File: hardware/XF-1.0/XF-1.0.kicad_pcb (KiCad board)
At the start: 2 copper layers, 121.3 x 99.7 mm, 16 parts

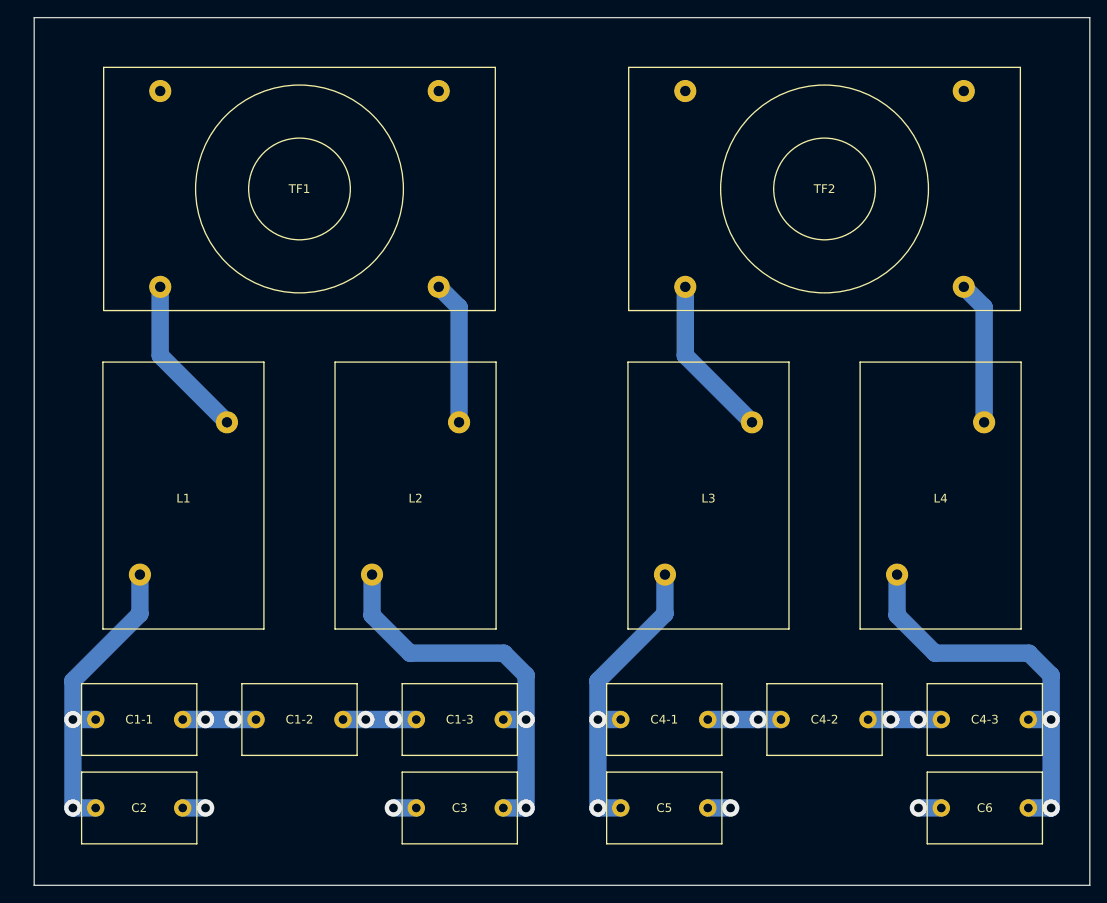
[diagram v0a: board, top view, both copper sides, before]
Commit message: modified:   Ferrite Transformer Calculation.xlsx 	modified:   README.md 	deleted:    hardware/XF-1.0/XF-1.0-backups/XF-1.0-2025-07-15_095716.zip 	new file:   hardware/XF-1.0/XF-1.0-backups/XF-1.0-2025-07-15_145509.zip 	new file:   hardware/XF-1.0/XF-1.0-backups/XF-1.0-2025-07-15_150114.zip 	new file:   hardware/XF-1.0/XF-1.0-backups/XF-1.0-2025-07-15_150614.zip 	new file:   hardware/XF-1.0/XF-1.0-backups/XF-1.0-2025-07-15_151503.zip 	new file:   hardware/XF-1.0/XF-1.0-backups/XF-1.0-2025-07-15_152320.zip 	new file:   hardware/XF-1.0/XF-1.0-backups/XF-1.0-2025-07-15_154638.zip 	modified:   hardware/XF-1.0/XF-1.0.kicad_pcb 	modified:   hardware/XF-1.0/XF-1.0.kicad_prl 	modified:   hardware/XF-1.0/XF-1.0.kicad_pro 	modified:   hardware/XF-1.0/XF-1.0.kicad_sch 	modified:   hardware/XF-1.0/_autosave-XF-1.0.kicad_sch 	modified:   hardware/XF-1.0/fp-info-cache
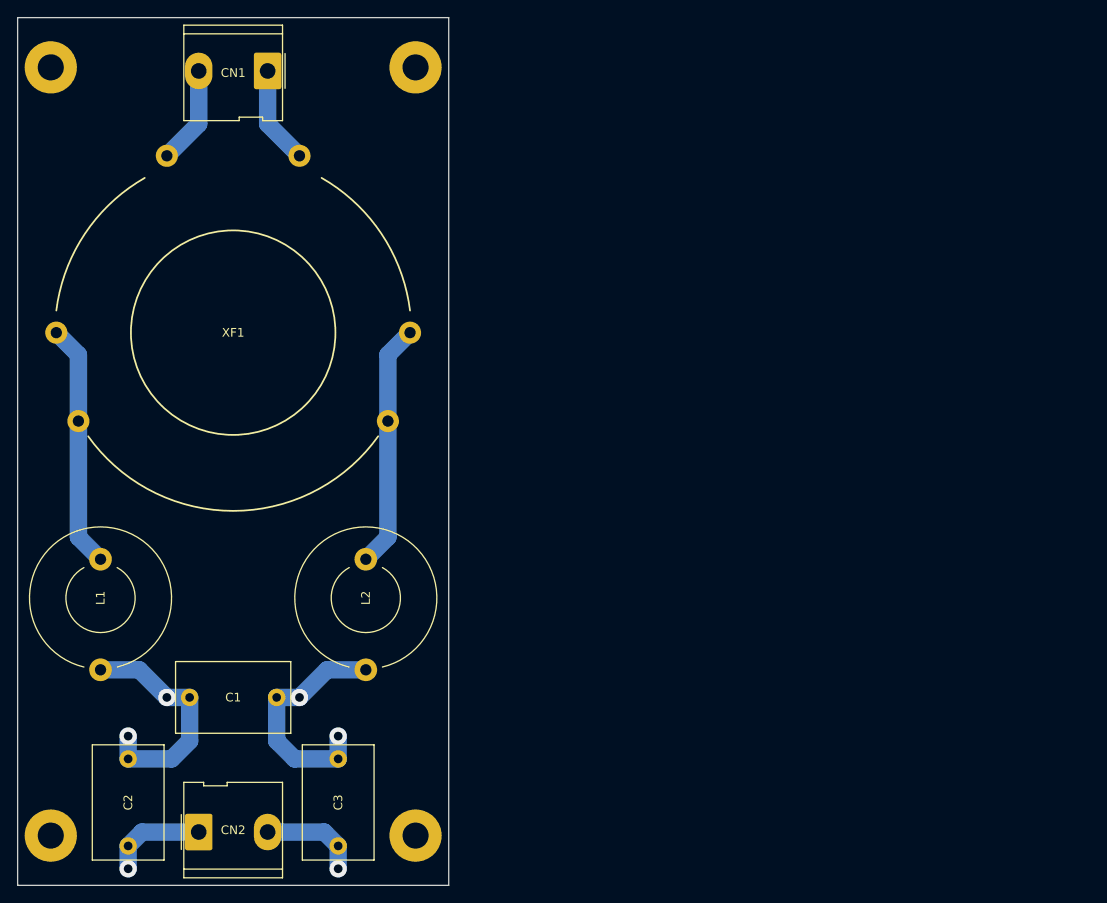
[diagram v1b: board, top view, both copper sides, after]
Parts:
- removed C1-1, C1-2, C1-3, C4-1, C4-2, C4-3: 1nF, Capacitor_THT:C_Rect_L13.0mm_W8.0mm_P10.00mm_FKS3_FKP3_MKS4
- removed C5, C6: 4.7nF, Capacitor_THT:C_Rect_L13.0mm_W8.0mm_P10.00mm_FKS3_FKP3_MKS4
- removed L3, L4: ~, Transformer_THT:Inductor-EE25
- removed TF1, TF2: ~, Transformer_THT:EE35-1P-1S-Vertical-2143
- added C1: 2.7nF, Capacitor_THT:C_Rect_L13.0mm_W8.0mm_P10.00mm_FKS3_FKP3_MKS4, F.Cu at (43.3, 124.5)
- added CN1: Conn_01x02, Connector_Molex:Molex_KK-396_5273-03A_1x03_P3.96mm_Vertical_2, F.Cu at (52.2, 52.5)
- added CN2: Conn_01x02, Connector_Molex:Molex_KK-396_5273-03A_1x03_P3.96mm_Vertical_2, F.Cu at (44.3, 139.9)
- added H1: ~, MountingHole:MountingHole_3mm_Pad, F.Cu at (27.3, 52.1)
- added H2: ~, MountingHole:MountingHole_3mm_Pad, F.Cu at (69.2, 52.1)
- added H3: ~, MountingHole:MountingHole_3mm_Pad, F.Cu at (27.3, 140.3)
- added H4: ~, MountingHole:MountingHole_3mm_Pad, F.Cu at (69.2, 140.3)
- added XF1: ~, Transformer_THT:Transformer_Toroid_Horizontal_OD40_ID23_H15, F.Cu at (48.3, 82.5)
- L1, L2: value ~ -> 29µH; footprint Transformer_THT:Inductor-EE25 -> Inductor_THT:L_Radial_Multilayer_D8.0mm_P12.70mm
- moved C3 19.8 mm to (60.3, 131.5), turned to -90 degrees
- moved L1 14.9 mm to (33.0, 113.0), turned to -90 degrees
- moved L2 12.8 mm to (63.5, 113.0), turned to -90 degrees
- moved C2 6.76 mm to (36.2, 131.5), turned to -90 degrees
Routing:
- net Net-(C4-3-Pad2): track 45.7 -> 0.00 mm, vias 2 -> 0
- net Net-(C4-1-Pad1): track 35.2 -> 0.00 mm, vias 2 -> 0
- net Net-(L3-Pad1): track 18.7 -> 0.00 mm
- net Net-(C1-Pad2): track 45.7 -> 27.1 mm
- net Net-(L4-Pad1): track 16.5 -> 0.00 mm
- net Net-(L2-Pad1): track 16.5 -> 28.1 mm
- net Net-(CN1-Pin_1): track 0.00 -> 11.3 mm
- net Net-(CN1-Pin_2): track 0.00 -> 11.3 mm
- net Net-(L1-Pad1): track 18.7 -> 28.1 mm
- net Net-(CN2-Pin_2): track 2.62 -> 11.4 mm
- net Net-(CN2-Pin_1): track 2.62 -> 11.4 mm
- net Net-(C4-2-Pad2): track 8.42 -> 0.00 mm, vias 2 -> 0
- net Net-(C1-2-Pad2): track 8.41 -> 0.00 mm, vias 2 -> 0
- net Net-(C1-1-Pad2): track 8.41 -> 0.00 mm, vias 2 -> 0
- net Net-(C4-1-Pad2): track 8.41 -> 0.00 mm, vias 2 -> 0
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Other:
- board size 121.3 x 99.7 mm -> 49.5 x 99.7 mm

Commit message: modified:   Ferrite Transformer Calculation.xlsx 	modified:   README.md 	deleted:    hardware/CTL-1.0/CTL-1.0-backups/CTL-1.0-2025-05-28_203223.zip 	new file:   hardware/CTL-1.0/CTL-1.0-backups/CTL-1.0-2025-07-16_143147.zip 	deleted:    hardware/PS-2.0/PS-2.0-backups/PS-2.0-2025-05-06_105341.zip 	new file:   hardware/PS-2.0/PS-2.0-backups/PS-2.0-2025-07-17_090338.zip 	deleted:    hardware/XF-1.0/#auto_saved_files# 	deleted:    hardware/XF-1.0/XF-1.0-backups/XF-1.0-2025-07-15_145509.zip 	new file:   hardware/XF-1.0/XF-1.0-backups/XF-1.0-2025-07-16_140719.zip 	new file:   hardware/XF-1.0/XF-1.0-backups/XF-1.0-2025-07-17_091914.zip 	new file:   hardware/XF-1.0/XF-1.0-backups/XF-1.0-2025-07-17_092825.zip 	new file:   hardware/XF-1.0/XF-1.0-backups/XF-1.0-2025-07-17_093426.zip 	new file:   hardware/XF-1.0/XF-1.0-backups/XF-1.0-2025-07-17_103845.zip 	new file:   hardware/XF-1.0/XF-1.0-backups/XF-1.0-2025-07-17_105026.zip 	new file:   hardware/XF-1.0/XF-1.0-backups/XF-1.0-2025-07-17_105651.zip 	modified:   hardware/XF-1.0/XF-1.0.kicad_pcb 	modified:   hardware/XF-1.0/XF-1.0.kicad_pro 	modified:   hardware/XF-1.0/XF-1.0.kicad_sch 	deleted:    hardware/XF-1.0/_autosave-XF-1.0.kicad_sch 	modified:   hardware/XF-1.0/fp-info-cache 	modified:   log.md
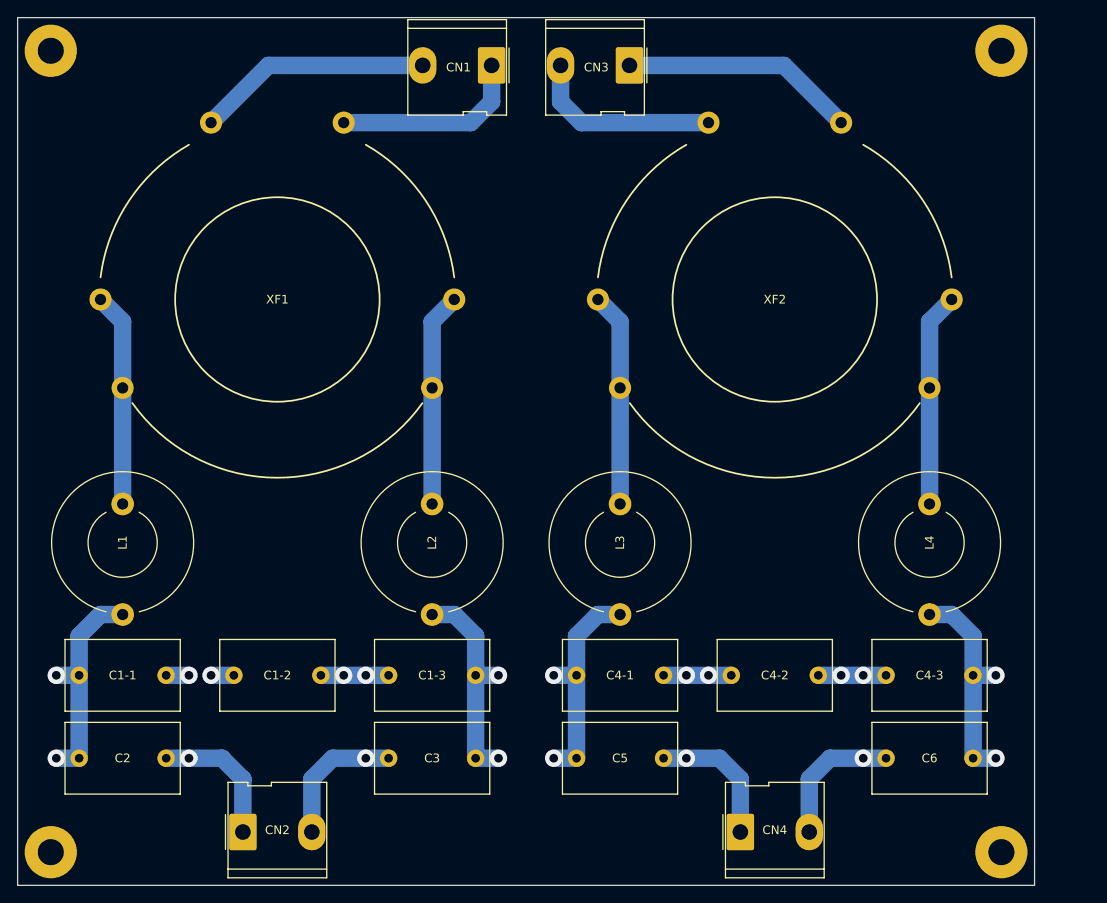
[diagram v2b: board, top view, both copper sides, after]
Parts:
- added C1-1: 2.7nF, Capacitor_THT:C_Rect_L13.0mm_W8.0mm_P10.00mm_FKS3_FKP3_MKS4, F.Cu at (30.6, 121.9)
- added C1-3: 2.7nF, Capacitor_THT:C_Rect_L13.0mm_W8.0mm_P10.00mm_FKS3_FKP3_MKS4, F.Cu at (66.1, 121.9)
- added C4-1: 2.7nF, Capacitor_THT:C_Rect_L13.0mm_W8.0mm_P10.00mm_FKS3_FKP3_MKS4, F.Cu at (87.7, 121.9)
- added C4-2: 2.7nF, Capacitor_THT:C_Rect_L13.0mm_W8.0mm_P10.00mm_FKS3_FKP3_MKS4, F.Cu at (105.5, 121.9)
- added C4-3: 2.7nF, Capacitor_THT:C_Rect_L13.0mm_W8.0mm_P10.00mm_FKS3_FKP3_MKS4, F.Cu at (123.3, 121.9)
- added C5: 4.7nF, Capacitor_THT:C_Rect_L13.0mm_W8.0mm_P10.00mm_FKS3_FKP3_MKS4, F.Cu at (87.7, 131.4)
- added C6: 4.7nF, Capacitor_THT:C_Rect_L13.0mm_W8.0mm_P10.00mm_FKS3_FKP3_MKS4, F.Cu at (133.3, 131.4)
- added CN3: Conn_01x02, Connector_Molex:Molex_KK-396_5273-03A_1x03_P3.96mm_Vertical_2, F.Cu at (93.8, 51.8)
- added CN4: Conn_01x02, Connector_Molex:Molex_KK-396_5273-03A_1x03_P3.96mm_Vertical_2, F.Cu at (106.5, 139.9)
- added L3: 29µH, Inductor_THT:L_Radial_Multilayer_D8.0mm_P12.70mm, F.Cu at (92.7, 106.7)
- added L4: 29µH, Inductor_THT:L_Radial_Multilayer_D8.0mm_P12.70mm, F.Cu at (128.3, 106.7)
- added XF2: ~, Transformer_THT:Transformer_Toroid_Horizontal_OD40_ID23_H15, F.Cu at (110.5, 78.7)
- moved H2 67.3 mm to (136.5, 50.2)
- moved H4 67.3 mm to (136.5, 142.2)
- moved CN1 25.7 mm to (78.0, 51.8)
- moved C3 15.8 mm to (76.1, 131.4), turned to 180 degrees
- moved L2 9.92 mm to (71.1, 106.7)
- moved L1 6.84 mm to (35.6, 106.7)
- moved XF1 6.35 mm to (53.3, 78.7)
- moved C1-2 5.68 mm to (48.3, 121.9)
- moved C2 5.64 mm to (30.6, 131.4), turned to 0 degrees
- moved CN2 5.08 mm to (49.4, 139.9)
- moved H1 1.91 mm to (27.3, 50.2)
- moved H3 1.91 mm to (27.3, 142.2)
- renumbered C1 to C1-2
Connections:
- C1-2 pad 1: Net-(C1-Pad1) -> Net-(C1-1-Pad2)
- C1-2 pad 2: Net-(C1-Pad2) -> Net-(C1-2-Pad2)
- C2 pad 1: Net-(C1-Pad1) -> Net-(C1-1-Pad1)
- C3 pad 1: Net-(C1-Pad2) -> Net-(C1-3-Pad2)
- L1 pad 2: Net-(C1-Pad1) -> Net-(C1-1-Pad1)
- L2 pad 2: Net-(C1-Pad2) -> Net-(C1-3-Pad2)
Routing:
- net Net-(C1-Pad2): track 27.1 -> 0.00 mm, vias 2 -> 0
- net Net-(C1-Pad1): track 27.1 -> 0.00 mm, vias 2 -> 0
- net Net-(CN3-Pin_1): track 0.00 -> 27.0 mm
- net Net-(C1-1-Pad1): track 0.00 -> 25.3 mm, vias 0 -> 2
- net Net-(C4-1-Pad1): track 0.00 -> 25.3 mm, vias 0 -> 2
- net Net-(C1-3-Pad2): track 0.00 -> 25.3 mm, vias 0 -> 2
- net Net-(C4-3-Pad2): track 0.00 -> 25.3 mm, vias 0 -> 2
- net Net-(L4-Pad1): track 0.00 -> 24.5 mm
- net Net-(L3-Pad1): track 0.00 -> 24.5 mm
- net Net-(CN3-Pin_2): track 0.00 -> 22.2 mm
- net Net-(CN4-Pin_1): track 0.00 -> 15.9 mm, vias 0 -> 1
- net Net-(CN4-Pin_2): track 0.00 -> 15.9 mm, vias 0 -> 1
- net Net-(CN1-Pin_2): track 11.3 -> 27.0 mm
- net Net-(CN1-Pin_1): track 11.3 -> 22.2 mm
- net Net-(C4-2-Pad2): track 0.00 -> 7.78 mm, vias 0 -> 2
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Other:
- board size 49.5 x 99.7 mm -> 116.8 x 99.7 mm
